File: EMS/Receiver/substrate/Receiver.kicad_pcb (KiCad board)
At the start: 2 copper layers, 81.3 x 61 mm, 17 parts, among them SW1 SW_SPDT, U1 LTV-817

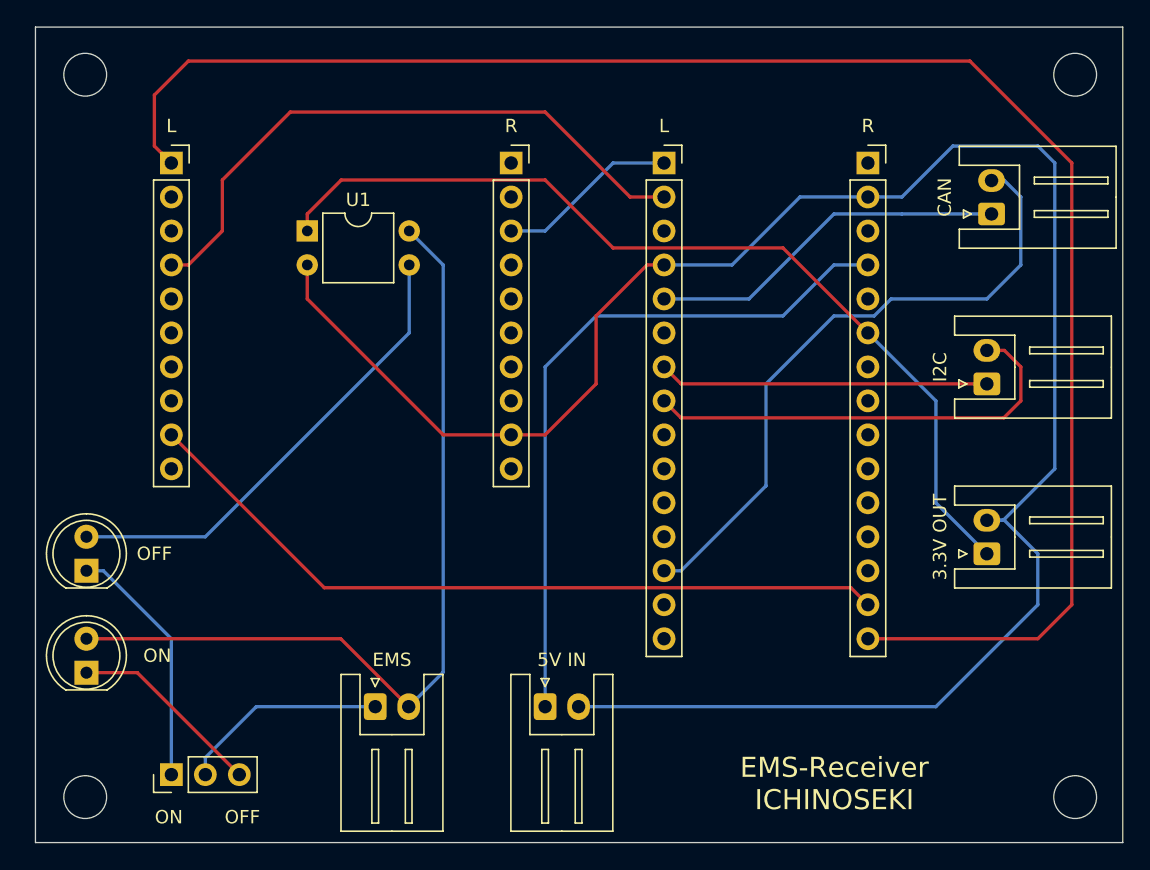
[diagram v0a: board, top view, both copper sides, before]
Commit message: Update Receiver.
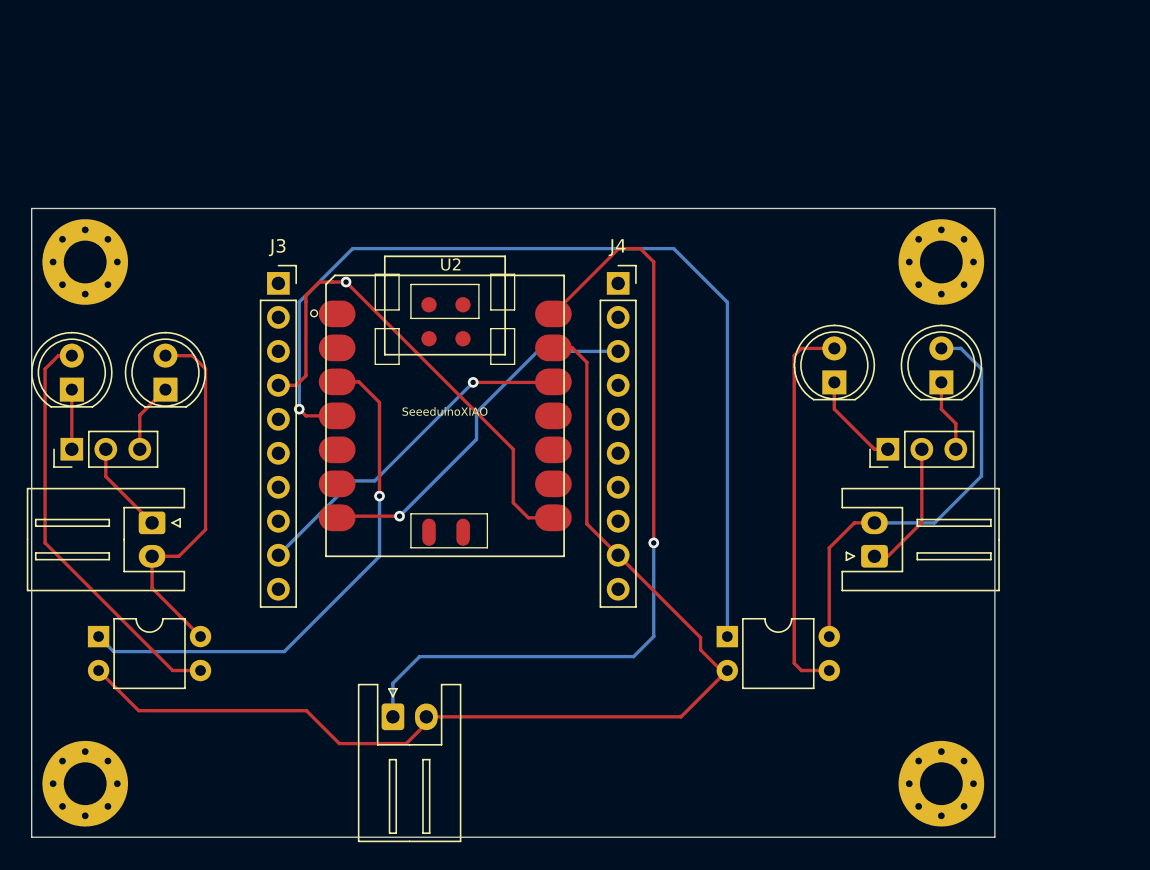
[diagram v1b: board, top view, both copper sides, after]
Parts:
- removed 3.3V OUT: 3V3_OUT, Connector_JST:JST_XH_S2B-XH-A_1x02_P2.50mm_Horizontal
- removed CAN: CAN, Connector_JST:JST_XH_S2B-XH-A_1x02_P2.50mm_Horizontal
- removed I2C: I2C, Connector_JST:JST_XH_S2B-XH-A_1x02_P2.50mm_Horizontal
- removed L: F303k8_Left, Connector_PinSocket_2.54mm:PinSocket_1x15_P2.54mm_Vertical
- removed R: F303k8_Right, Connector_PinSocket_2.54mm:PinSocket_1x15_P2.54mm_Vertical
- removed the REF** at (159.0, 149.0)
- removed the REF** at (159.0, 95.0)
- removed the REF** at (85.0, 95.0)
- removed the REF** at (85.0, 149.0)
- added D3: LED, LED_THT:LED_D5.0mm, F.Cu at (141.0, 118.0)
- added D4: LED, LED_THT:LED_D5.0mm, F.Cu at (149.0, 118.0)
- added J1: RESS_OUT2, Connector_JST:JST_XH_S2B-XH-A_1x02_P2.50mm_Horizontal, F.Cu at (144.0, 131.0)
- added REF**: MountingHole_3.2mm_M3_Pad_Via, MountingHole:MountingHole_3.2mm_M3_Pad_Via, F.Cu at (149.0, 148.0)
- added REF**: MountingHole_3.2mm_M3_Pad_Via, MountingHole:MountingHole_3.2mm_M3_Pad_Via, F.Cu at (149.0, 109.0)
- added REF**: MountingHole_3.2mm_M3_Pad_Via, MountingHole:MountingHole_3.2mm_M3_Pad_Via, F.Cu at (85.0, 109.0)
- added REF**: MountingHole_3.2mm_M3_Pad_Via, MountingHole:MountingHole_3.2mm_M3_Pad_Via, F.Cu at (85.0, 148.0)
- added SW2: SW_SPDT, Connector_PinHeader_2.54mm:PinHeader_1x03_P2.54mm_Vertical, F.Cu at (145.0, 123.0)
- added U2: SeeeduinoXIAO, Seeeduino XIAO KICAD:Seeeduino XIAO-MOUDLE14P-2.54-21X17.8MM, F.Cu at (103.0, 131.0)
- added U3: LTV-817, Package_DIP:DIP-4_W7.62mm, F.Cu at (133.0, 137.0)
- J3: renamed from L; value ADP_Left -> ADP_L
- J4: renamed from R; value ADP_Right -> ADP_R
- J5: renamed from 5V IN
- J6: renamed from EMS; value EMS_OUT -> RESS_OUT1
- moved U1 34.1 mm to (86.0, 137.0)
- moved SW1 25.4 mm to (84.0, 123.0)
- moved D2 22.0 mm to (91.0, 118.5)
- moved J6 21.6 mm to (90.0, 128.5), turned to 270 degrees
- moved D1 13.6 mm to (84.0, 118.5)
- moved J3 12.0 mm to (99.4, 110.6)
- moved J4 12.0 mm to (124.8, 110.6)
- moved J5 11.4 mm to (108.0, 143.0)
- renumbered OFF to D1, ON to D2
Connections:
- J3 pad 1: Net-(J2-Pad15) -> (no net)
- J3 pad 10: Net-(J3-Pad10) -> (no net)
- J3 pad 2: Net-(J3-Pad2) -> (no net)
- J3 pad 3: Net-(J3-Pad3) -> (no net)
- J3 pad 4: Net-(J1-Pad2) -> RX
- J3 pad 5: Net-(J3-Pad5) -> (no net)
- J3 pad 6: Net-(J3-Pad6) -> (no net)
- J3 pad 7: Net-(J3-Pad7) -> (no net)
- J3 pad 8: Net-(J3-Pad8) -> (no net)
- J3 pad 9: Net-(J2-Pad14) -> +3V3
- J4 pad 1: Net-(J4-Pad1) -> (no net)
- J4 pad 10: Net-(J4-Pad10) -> (no net)
- J4 pad 2: Net-(J4-Pad2) -> (no net)
- J4 pad 3: Net-(J1-Pad1) -> TX
- J4 pad 4: Net-(J4-Pad4) -> (no net)
- J4 pad 5: Net-(J4-Pad5) -> (no net)
- J4 pad 6: Net-(J4-Pad6) -> (no net)
- J4 pad 7: Net-(J4-Pad7) -> (no net)
- J4 pad 8: Net-(J4-Pad8) -> (no net)
- U1 pad 1: Net-(J10-Pad1) -> Out1
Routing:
- net Net-(J2-Pad15): track 127.7 -> 0.00 mm
- net Out2: track 0.00 -> 71.4 mm, vias 0 -> 1
- net Net-(J10-Pad1): track 69.2 -> 0.00 mm
- net GND: track 150.7 -> 82.4 mm
- net Net-(J2-Pad14): track 57.3 -> 0.00 mm
- net Net-(J1-Pad13): track 48.4 -> 0.00 mm
- net Net-(J1-Pad2): track 46.4 -> 0.00 mm
- net Out1: track 0.00 -> 39.7 mm, vias 0 -> 1
- net RX: track 0.00 -> 36.9 mm, vias 0 -> 1
- net Net-(D2-Pad2): track 63.9 -> 27.7 mm
- net Net-(J1-Pad8): track 33.3 -> 0.00 mm
- net Net-(D4-Pad2): track 0.00 -> 31.9 mm
- net Net-(D3-Pad2): track 0.00 -> 29.1 mm
- net TX: track 0.00 -> 27.3 mm, vias 0 -> 1
- net Net-(J1-Pad5): track 27.1 -> 0.00 mm
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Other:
- board size 81.3 x 61 mm -> 72 x 47 mm
- board text removed: "EMS-Receiver ICHINOSEKI"
- board text removed: "OFF"
- board text removed: "ON"
